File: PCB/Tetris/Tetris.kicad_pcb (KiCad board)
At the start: 2 copper layers, 135 x 56 mm, 51 parts, among them J1 Power, J2 PWM, J3 Analog, J4 PWM, J5 Analog, J6 Communication, J7 Digital, M1 RGBMatrix, M2 RGBMatrix, SW1 SW_Push, SW2 SW_Push, SW3 SW_Push, SW4 SW_Push, SW5 SW_Push, SW6 SW_Push, SW7 SW_Push, U1 74HC595, U2 74HC595

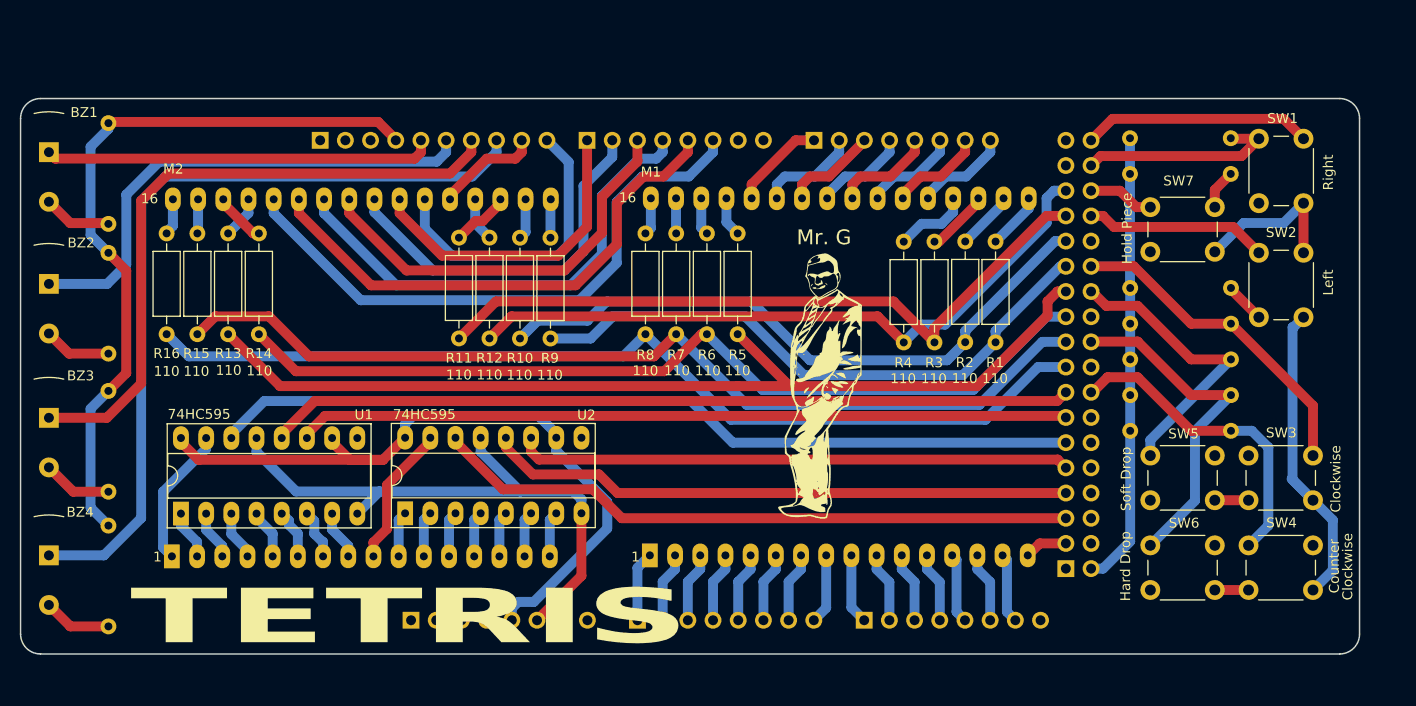
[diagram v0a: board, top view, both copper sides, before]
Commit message: MASSIVE PROGRESS
Redesign PCB to use ports
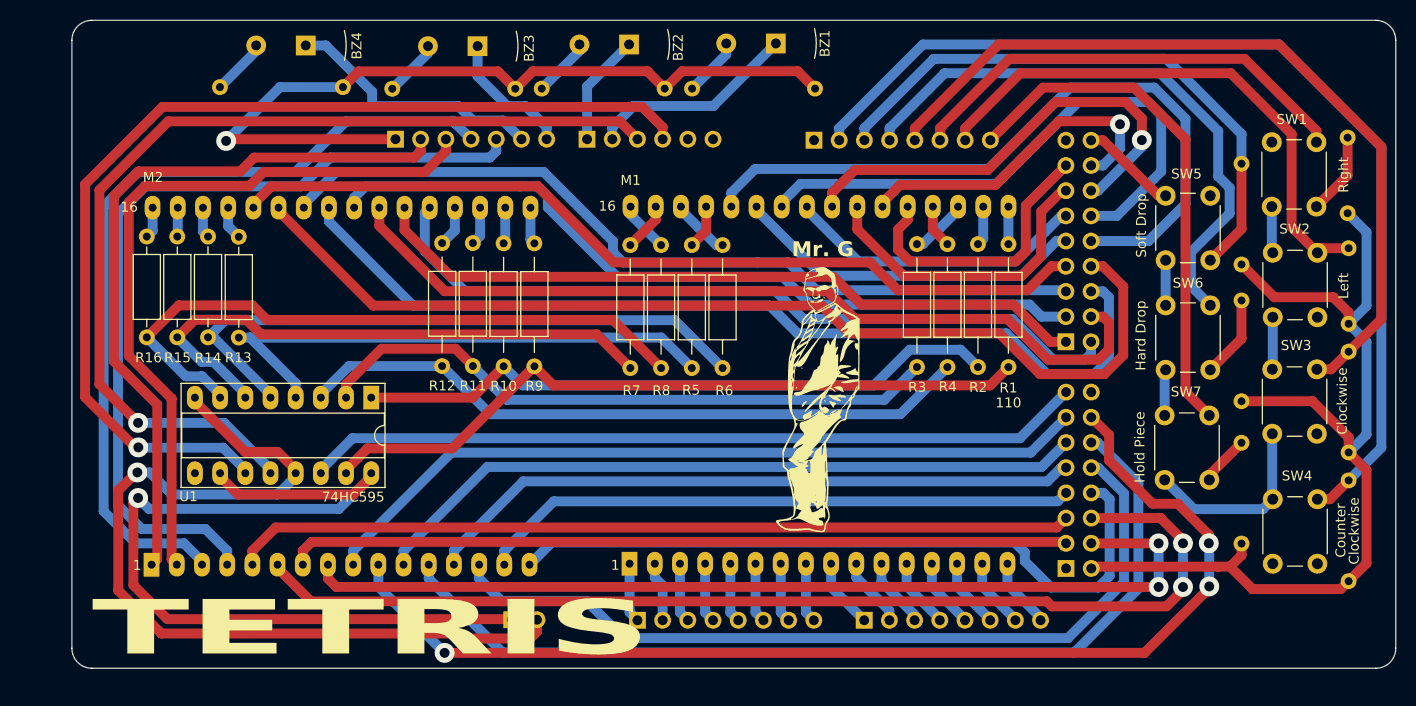
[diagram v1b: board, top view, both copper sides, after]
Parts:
- removed U2: 74HC595, Package_DIP:DIP-16_W7.62mm_Socket_LongPads
- added J8: Digital, Connector_PinHeader_2.54mm:PinHeader_2x08_P2.54mm_Vertical, B.Cu at (188.4, 125.4)
- G2: renamed from Mr. G
- J1: footprint Connector_PinHeader_2.54mm:PinHeader_1x08_P2.54mm_Vertical -> Connector_PinHeader_2.54mm:PinHeader_1x02_P2.54mm_Vertical
- J2: footprint Connector_PinHeader_2.54mm:PinHeader_1x10_P2.54mm_Vertical -> Connector_PinHeader_2.54mm:PinHeader_1x07_P2.54mm_Vertical
- J4: footprint Connector_PinHeader_2.54mm:PinHeader_1x08_P2.54mm_Vertical -> Connector_PinHeader_2.54mm:PinHeader_1x06_P2.54mm_Vertical
- J7: footprint Connector_PinHeader_2.54mm:PinHeader_2x18_P2.54mm_Vertical -> Connector_PinHeader_2.54mm:PinHeader_2x09_P2.54mm_Vertical
- R1, R10, R11, R12, R2, R24, R25, R26, R27, R3, R4, R5, R6, R7, R8, R9: footprint Resistor_THT:R_Axial_DIN0207_L6.3mm_D2.5mm_P10.16mm_Horizontal -> RGBMatrix:R_Axial_DIN0207_L6.3mm_D2.5mm_P12.40mm_Horizontal
- R17, R18: footprint Resistor_THT:R_Axial_DIN0207_L6.3mm_D2.5mm_P10.16mm_Horizontal -> Resistor_THT:R_Axial_DIN0207_L6.3mm_D2.5mm_P7.62mm_Horizontal
- moved BZ1 74.1 mm to (159.2, 72.5), turned to 180 degrees
- moved R24 70.1 mm to (161.9, 77.0), turned to 180 degrees
- moved BZ2 63.3 mm to (144.3, 72.5), turned to 180 degrees
- moved BZ4 57.6 mm to (111.8, 72.7), turned to 180 degrees
- moved R25 57.3 mm to (146.7, 77.0), turned to 180 degrees
- moved BZ3 57.2 mm to (129.1, 72.7), turned to 180 degrees
- moved R26 50.1 mm to (131.7, 77.0), turned to 180 degrees
- moved R27 49.6 mm to (114.3, 76.8), turned to 180 degrees
- moved R23 27.1 mm to (206.1, 112.7), turned to -90 degrees
- moved SW5 26.9 mm to (202.9, 87.8), turned to -90 degrees
- moved R20 26.7 mm to (216.9, 126.7), turned to 90 degrees
- moved R19 25.6 mm to (216.9, 113.7), turned to 90 degrees
- moved SW6 24.9 mm to (202.9, 98.8), turned to -90 degrees
- moved R17 23.2 mm to (216.8, 89.6), turned to 90 degrees
- moved J7 22.9 mm to (188.4, 102.5)
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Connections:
- BZ1 pad 1: /*13 -> /*6
- BZ2 pad 1: /*12 -> /*7
- BZ3 pad 1: /*11 -> /*8
- BZ4 pad 1: /*10 -> /*9
- J1 pad 1: unconnected-(J1-Pin_1-Pad1) -> +5V
- J1 pad 2: /IOREF -> GND
- J2 pad 1: /SCL/21 -> GND
- J2 pad 2: /SDA/20 -> /*13
- J2 pad 3: /AREF -> /*12
- J2 pad 4: GND -> /*11
- J2 pad 5: /*13 -> /*10
- J2 pad 6: /*12 -> /*9
- J2 pad 7: /*11 -> /*8
- J6 pad 1: /TX3/14 -> /14
- J6 pad 2: /RX3/15 -> /15
- J6 pad 3: /TX2/16 -> /16
- J6 pad 4: /RX2/17 -> /17
- J6 pad 5: /TX1/18 -> /18
- J6 pad 6: /RX1/19 -> /19
- J6 pad 7: /SDA/20 -> /20
- J6 pad 8: /SCL/21 -> /21
- J7 pad 1: GND -> /36
- J7 pad 10: /47 -> /29
- J7 pad 11: /*44 -> /26
- J7 pad 12: /*45 -> /27
- J7 pad 13: /42 -> /24
- J7 pad 14: /43 -> /25
- J7 pad 15: /40 -> /22
- J7 pad 16: /41 -> /23
- J7 pad 17: /38 -> +5V
- J7 pad 18: /39 -> +5V
- J7 pad 2: GND -> /37
- J7 pad 3: /*52 -> /34
- J7 pad 4: /53 -> /35
- J7 pad 5: /50 -> /32
- J7 pad 6: /51 -> /33
- J7 pad 7: /48 -> /30
- J7 pad 8: /49 -> /31
- J7 pad 9: /*46 -> /28
- M1 pad 16: /*52 -> /A15
- M1 pad 21: /SCL/21 -> /22
- M1 pad 22: /SDA/20 -> /23
- M1 pad 23: /RX1/19 -> /24
- M1 pad 24: /TX1/18 -> /25
- M1 pad 25: /RX2/17 -> /26
- M1 pad 26: /TX2/16 -> /27
- M1 pad 27: /RX3/15 -> /28
- M1 pad 28: /TX3/14 -> /29
- M2 pad 1: /S1 -> /*13
- M2 pad 10: /S10 -> /43
- M2 pad 11: /S11 -> /*44
- M2 pad 12: /S12 -> /*45
- M2 pad 13: /S13 -> /*46
- M2 pad 14: /S14 -> /47
- M2 pad 15: /S15 -> /48
- M2 pad 16: /S16 -> /49
- M2 pad 2: /S2 -> /*12
- M2 pad 21: /*9 -> /37
- M2 pad 22: /*8 -> /36
- M2 pad 23: /*7 -> /35
- M2 pad 24: /*6 -> /34
- M2 pad 25: /*5 -> /33
- M2 pad 26: /*4 -> /32
- M2 pad 27: /*3 -> /31
- M2 pad 28: /*2 -> /30
- M2 pad 3: /S3 -> /*11
- M2 pad 4: /S4 -> /*10
- M2 pad 5: /S5 -> /50
- M2 pad 6: /S6 -> /51
- M2 pad 7: /S7 -> /*52
- M2 pad 8: /S8 -> /53
- M2 pad 9: /S9 -> /42
- R1 pad 1: /30 -> /S1
- R10 pad 1: /28 -> /S2
- R11 pad 1: /26 -> /S3
- R12 pad 1: /24 -> /S4
- R13 pad 2: /32 -> /S5
- R14 pad 2: /34 -> /S6
- R15 pad 2: /36 -> /S7
- R16 pad 2: /38 -> /S8
- R17 pad 2: /23 -> /19
- R18 pad 2: /27 -> /20
- R19 pad 2: /31 -> /18
- R2 pad 1: /28 -> /S2
- R20 pad 2: /41 -> /15
- R21 pad 2: /33 -> /16
- R22 pad 1: /37 -> /17
- R23 pad 1: /25 -> /21
- R3 pad 1: /26 -> /S3
- R4 pad 1: /24 -> /S4
- R5 pad 2: /32 -> /S5
- R6 pad 2: /34 -> /S6
- R7 pad 2: /36 -> /S7
- R8 pad 2: /38 -> /S8
- R9 pad 1: /30 -> /S1
- SW1 pad 1: /23 -> /19
- SW2 pad 1: /27 -> /20
- SW3 pad 1: /31 -> /18
- SW4 pad 1: /41 -> /15
- SW5 pad 1: /33 -> /16
- SW6 pad 1: /37 -> /17
- SW7 pad 1: /25 -> /21
- U1 pad 11: /42 -> /*4
- U1 pad 12: /40 -> /*5
- U1 pad 14: /*44 -> /40
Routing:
- net /43: track 0.00 -> 115.1 mm, vias 0 -> 3
- net /51: track 0.00 -> 109.1 mm, vias 0 -> 2
- net /15: track 0.00 -> 102.6 mm
- net /38: track 98.3 -> 0.00 mm
- net /53: track 0.00 -> 96.7 mm, vias 0 -> 2
- net /*45: track 0.00 -> 95.8 mm
- net GND: track 181.0 -> 272.7 mm, vias 0 -> 2
- net /35: track 0.00 -> 86.2 mm
- net /47: track 0.00 -> 84.6 mm
- net /18: track 0.00 -> 82.0 mm
- net /*52: track 4.34 -> 78.8 mm
- net /29: track 0.00 -> 72.5 mm
- net /49: track 0.00 -> 72.2 mm
- net /31: track 33.2 -> 104.1 mm
- net /17: track 0.00 -> 67.8 mm
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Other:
- board size 135 x 56 mm -> 133.5 x 65.3 mm
- board text added: "Jonathan Cai 2023 Thanks: Evan Tao"
- board text added: "Mr. G"
- board text removed: "Jonathan Cai 2023"
